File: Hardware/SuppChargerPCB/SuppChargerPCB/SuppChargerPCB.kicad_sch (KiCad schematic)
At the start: 62 parts, among them J1 SLIMSTACK, J2 SLIMSTACK, Q10 NMOS, Q7 NMOS, Q8 NMOS, Q9 NMOS, U1 BQ25756ERRVR

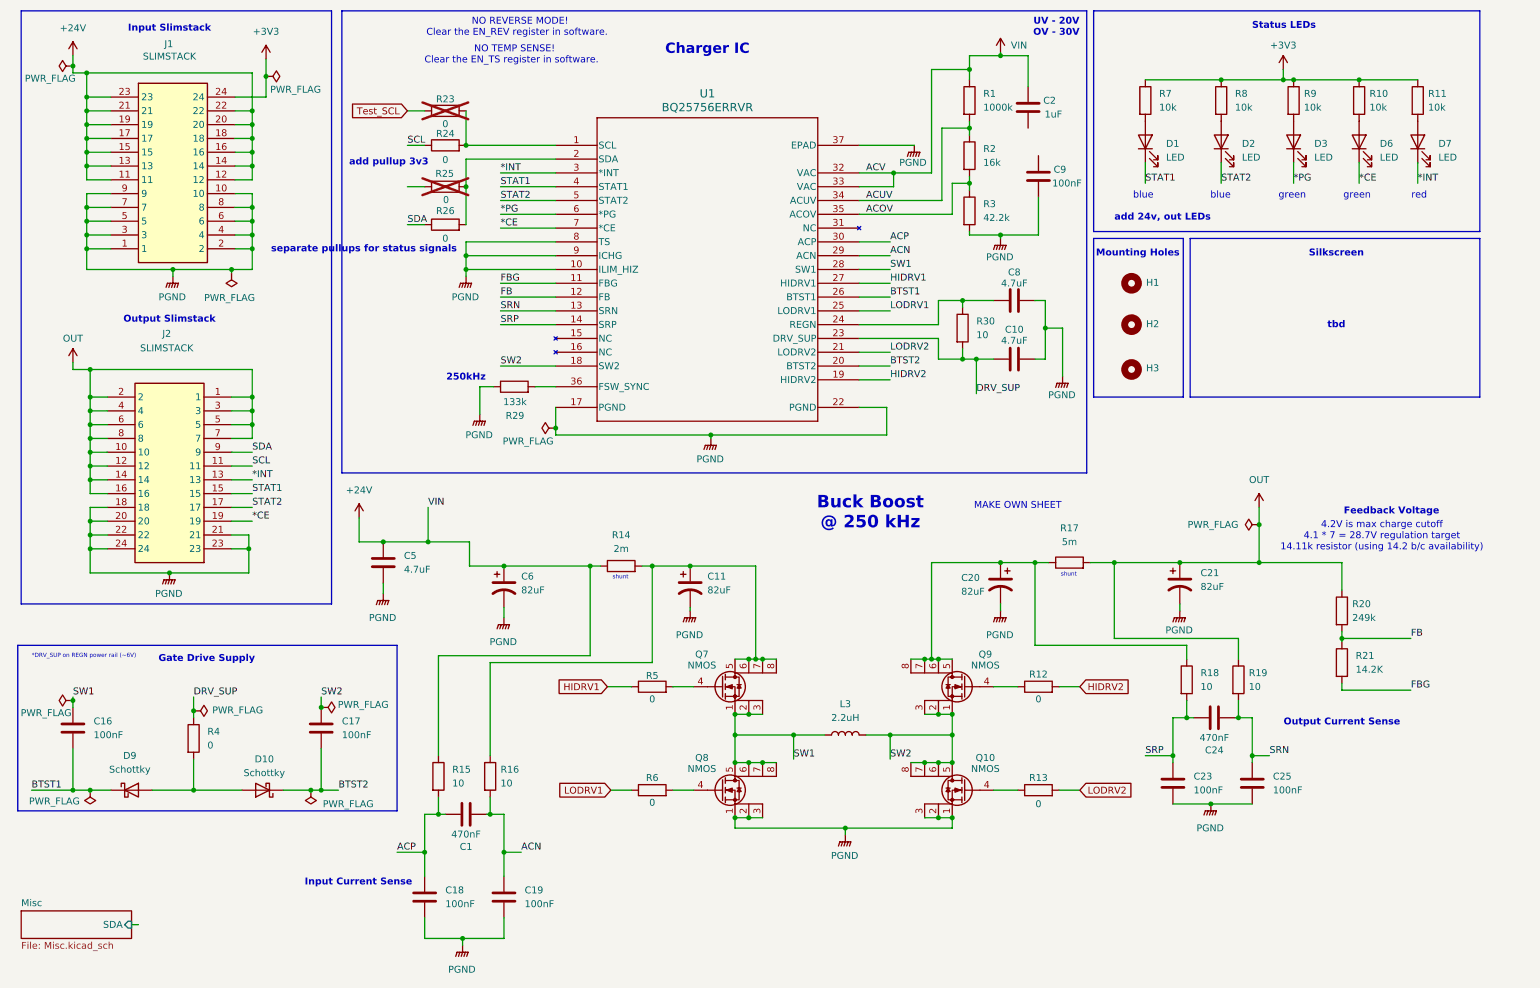
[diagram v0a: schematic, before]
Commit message: lakshay comments
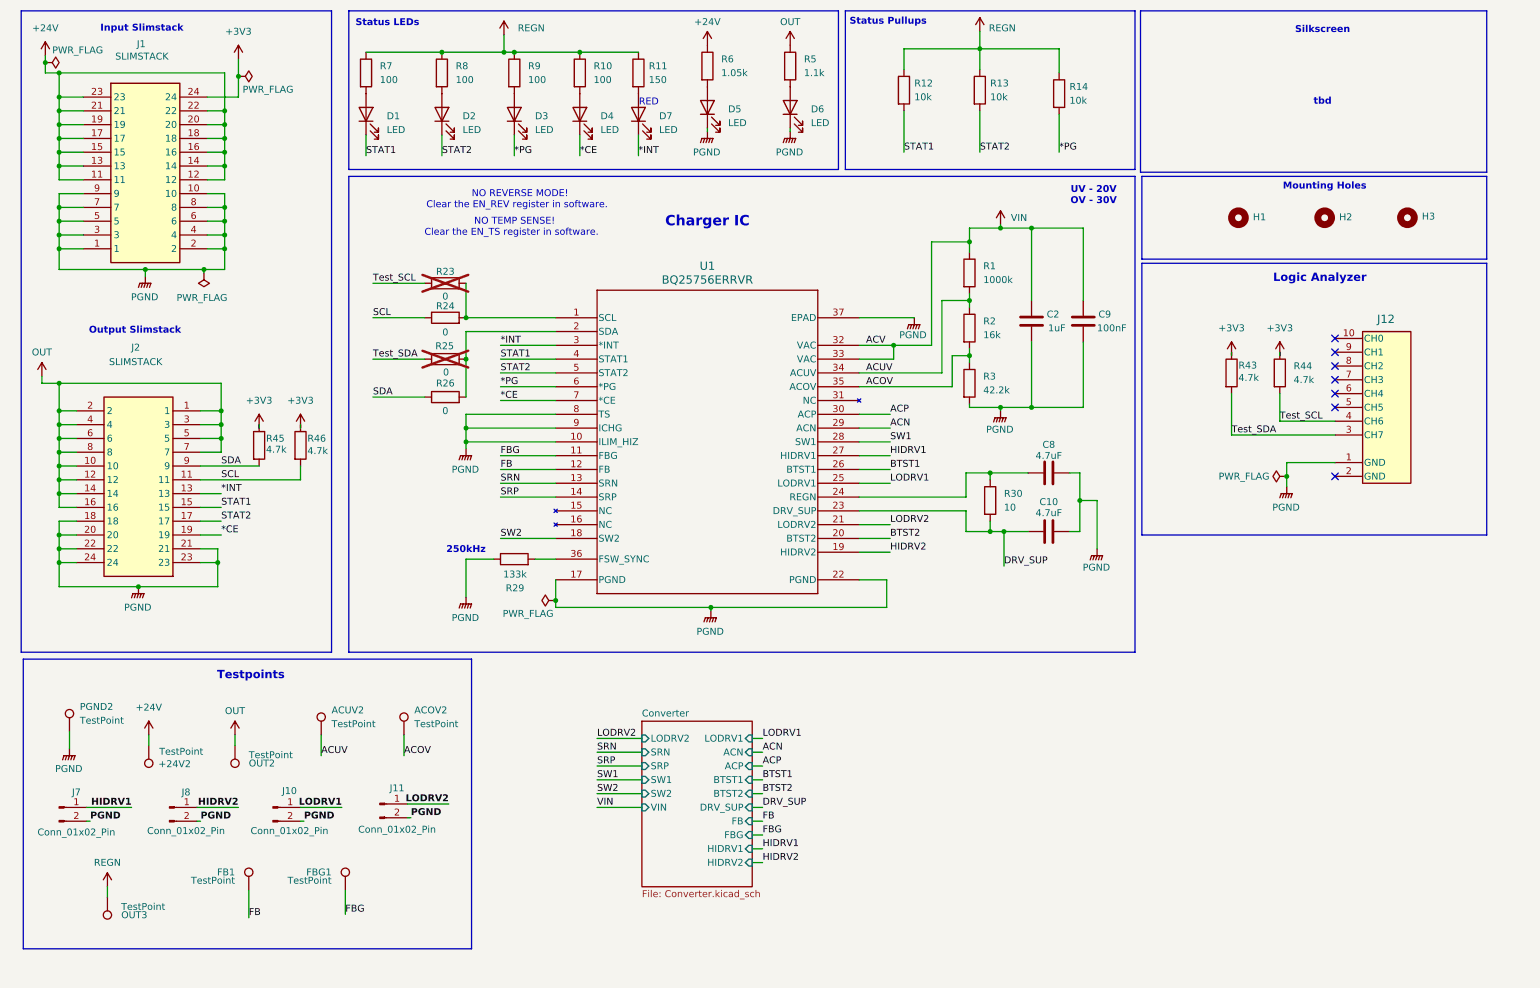
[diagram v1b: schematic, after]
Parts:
- removed C1, C24: 470nF, Capacitor_SMD:C_0603_1608Metric, symbol Device:C
- removed C11, C20, C21, C6: 82uF, Components:CAPAE830X1050N, symbol Device:C_Polarized_US
- removed C16, C17, C18, C19, C23, C25: 100nF, Capacitor_SMD:C_0603_1608Metric, symbol Device:C
- removed C5: 4.7uF, Capacitor_SMD:C_0805_2012Metric, symbol Device:C
- removed D10, D9: Schottky, Components:SOD3716X145N, symbol Device:D_Schottky
- removed L3: 2.2uH, Components:HCM1A0503V22R2R, symbol Device:L
- removed Q10, Q7, Q8, Q9: NMOS, symbol NMOS_Buck:SI3456DDV-T1-GE3
- removed R15, R16, R18, R19: 10, Resistor_SMD:R_0603_1608Metric, symbol Device:R
- removed R17: 5m, Resistor_SMD:R_0603_1608Metric, symbol Device:R
- removed R20: 249k, Resistor_SMD:R_0603_1608Metric, symbol Device:R
- removed R21: 14.2K, Resistor_SMD:R_0603_1608Metric, symbol Device:R
- removed R4: 0, Resistor_SMD:R_0603_1608Metric, symbol Device:R
- added +24V2, ACOV2, ACUV2, FB1, FBG1, OUT2, OUT3, PGND2: TestPoint, Connector_PinHeader_2.54mm:PinHeader_1x01_P2.54mm_Vertical, symbol Connector:TestPoint
- added D4, D5: LED, Diode_SMD:D_0603_1608Metric, symbol Device:LED
- added J10, J11, J7, J8: Conn_01x02_Pin, Connector_PinHeader_2.54mm:PinHeader_1x02_P2.54mm_Vertical, symbol Connector:Conn_01x02_Pin
- added J12: SFH11-PBPC-D05-ST-BK, UTSVT_Connectors:CONN_SFH11-xxxC-D05-ST-XX_SUL, symbol utsvt_connectors:SFH11-PBPC-D05-ST-BK
- added R43, R44, R45, R46: 4.7k, Resistor_SMD:R_0603_1608Metric, symbol Device:R
- D3, D6: P/N 150060GS75000 -> LTST-C193TBKT-5A
- R10, R7, R8, R9: value 10k -> 100; P/N CRCW060310K0FKEI -> AR0603FR-07100RL
- R11: value 10k -> 150; P/N CRCW060310K0FKEI -> AC0603JR-13150RL
- R12, R13: value 0 -> 10k; P/N (none) -> CRCW060310K0FKEI
- R14: value 2m -> 10k; P/N RV0603FR-072ML -> CRCW060310K0FKEI
- R5: value 0 -> 1.1k; P/N (none) -> MCT0603MD1101BP500
- R6: value 0 -> 1.05k; P/N (none) -> AR0603FR-071K05L
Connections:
- net *CE: now also D4.1 (K); no longer D6.1 (K)
- net *PG: now also R14.2
- net +24V: now also R6.1, +24V2.1; no longer C2.1, R1.1, R14.1, U1.32 (VAC), U1.33 (VAC)
- net +3V3: now also R43.1, R44.1, R45.1, R46.1; no longer R10.1, R11.1, R7.1, R8.1, R9.1
- net ACOV: now also ACOV2.1
- net ACUV: now also ACUV2.1
- net FB: now also FB1.1
- net FBG: now also FBG1.1
- net HIDRV1: now also J7.1 (Pin_1); no longer R5.1
- net HIDRV2: now also J8.1 (Pin_1); no longer R12.2
- net LODRV1: now also J10.1 (Pin_1); no longer R6.1
- net LODRV2: now also J11.1 (Pin_1); no longer R13.2
- net OUT: now also R5.1, OUT2.1
- net PGND: now also C2.2, D6.1 (K), D5.1 (K), J10.2 (Pin_2), J11.2 (Pin_2), J12.1 (GND), J7.2 (Pin_2), J8.2 (Pin_2), PGND2.1
- net SCL: now also R46.2
- net SDA: now also R45.2
- net STAT1: now also R12.2
- net STAT2: now also R13.2
- net Test_SCL: now also J12.4 (CH6), R44.2
- net at R5.2: now also D6.2 (A)
- net REGN: now reaches R13.1
- net REGN: now also R10.1, R11.1, R12.1, R14.1, R7.1, R8.1, R9.1, OUT3.1
- net at R10.2: now also D4.2 (A); no longer D6.2 (A)
- net VIN: now reaches C9.1
- net VIN: now also C2.1, R1.1, U1.32 (VAC), U1.33 (VAC)
- net at R6.2: now also D5.2 (A)
- net Test_SDA: now reaches R25.1
- net Test_SDA: now also J12.3 (CH7), R43.2
- no-connect marks 0 -> 7
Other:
- removed sheet Misc
- added sheet Converter (Converter.kicad_sch)
- note added: "Logic Analyzer"
- note added: "RED"
- note added: "Status Pullups"
- note added: "Testpoints"
- note removed: "*DRV_SUP on REGN power rail (~6V)"
- note removed: "4.2V is max charge cutoff 4.1 * 7 = 28.7V regulation target 14.11k resistor (using 14.2 b/c availability)"
- note removed: "Buck Boost @ 250 kHz"
- note removed: "Feedback Voltage"
- note removed: "Gate Drive Supply"
- note removed: "Input Current Sense"
- note removed: "MAKE OWN SHEET"
- note removed: "Output Current Sense"
- note removed: "add 24v, out LEDs"
- note removed: "add pullup 3v3"
- note removed: "blue"
- note removed: "green"
- note removed: "red"
- note removed: "separate pullups for status signals"
- note removed: "shunt"
- moved on the sheet: C10, C2, C8, C9, D1, D2, D7, H1, H2, H3, J1, J2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
